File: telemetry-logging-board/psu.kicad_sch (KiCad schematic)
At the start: 23 parts, among them U10 TPS22919DCK, U16 TPS22919DCK, U17 TPS22919DCK, U18 AP61300Z6, U8 AP61300Z6

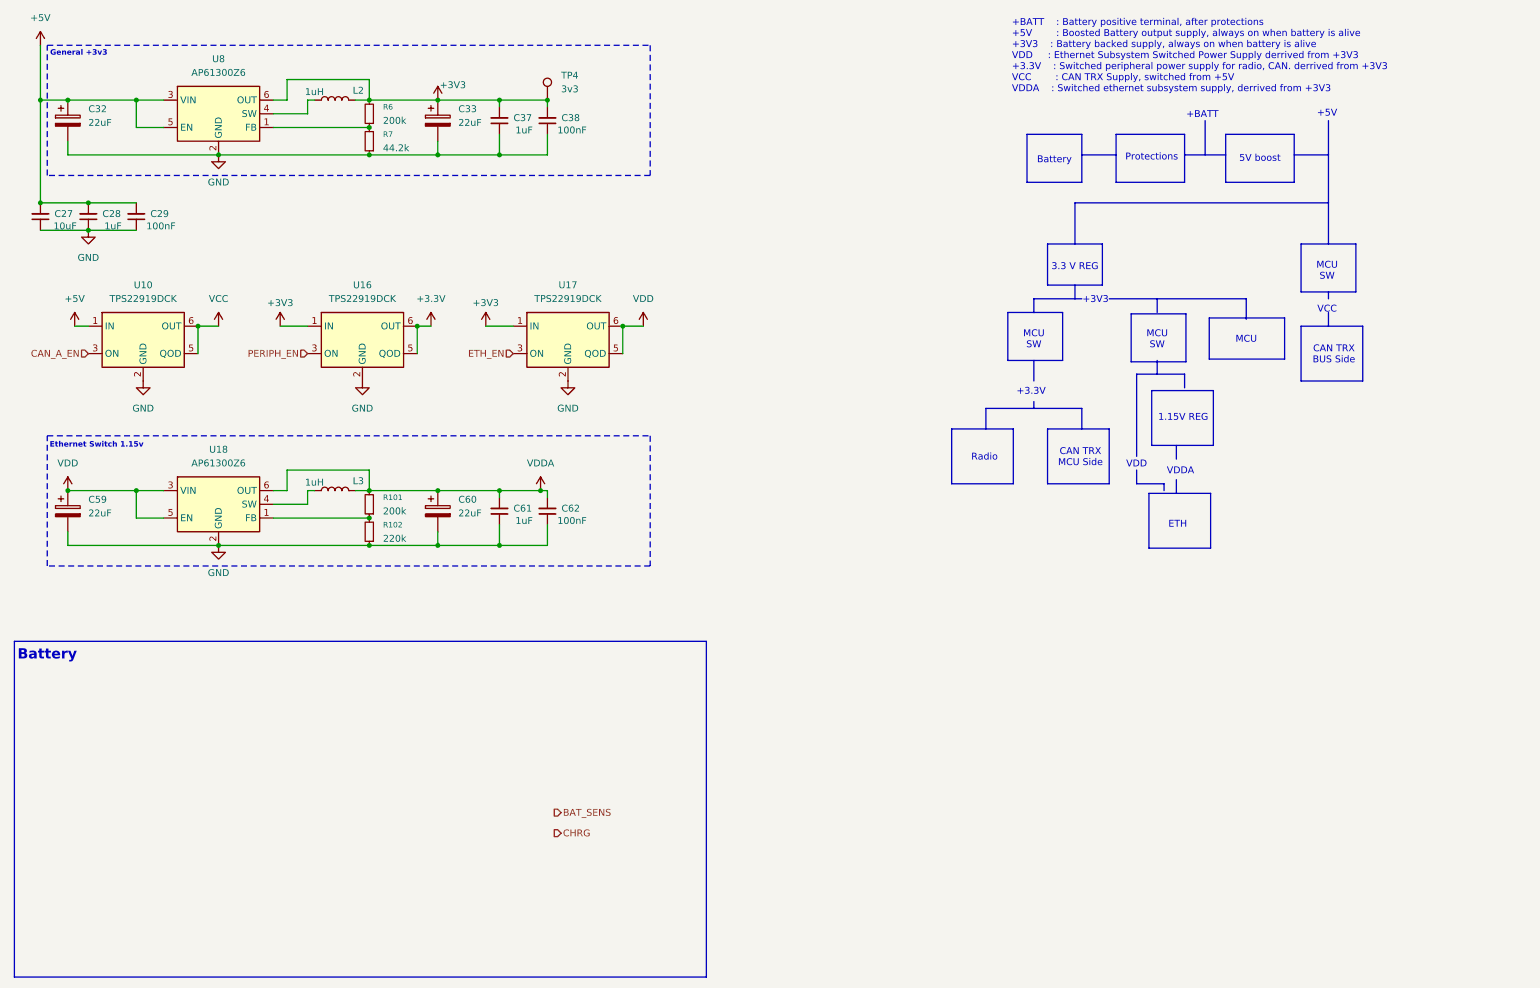
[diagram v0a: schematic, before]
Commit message: replace LR2021 with seeed wio LR2021, rework psu
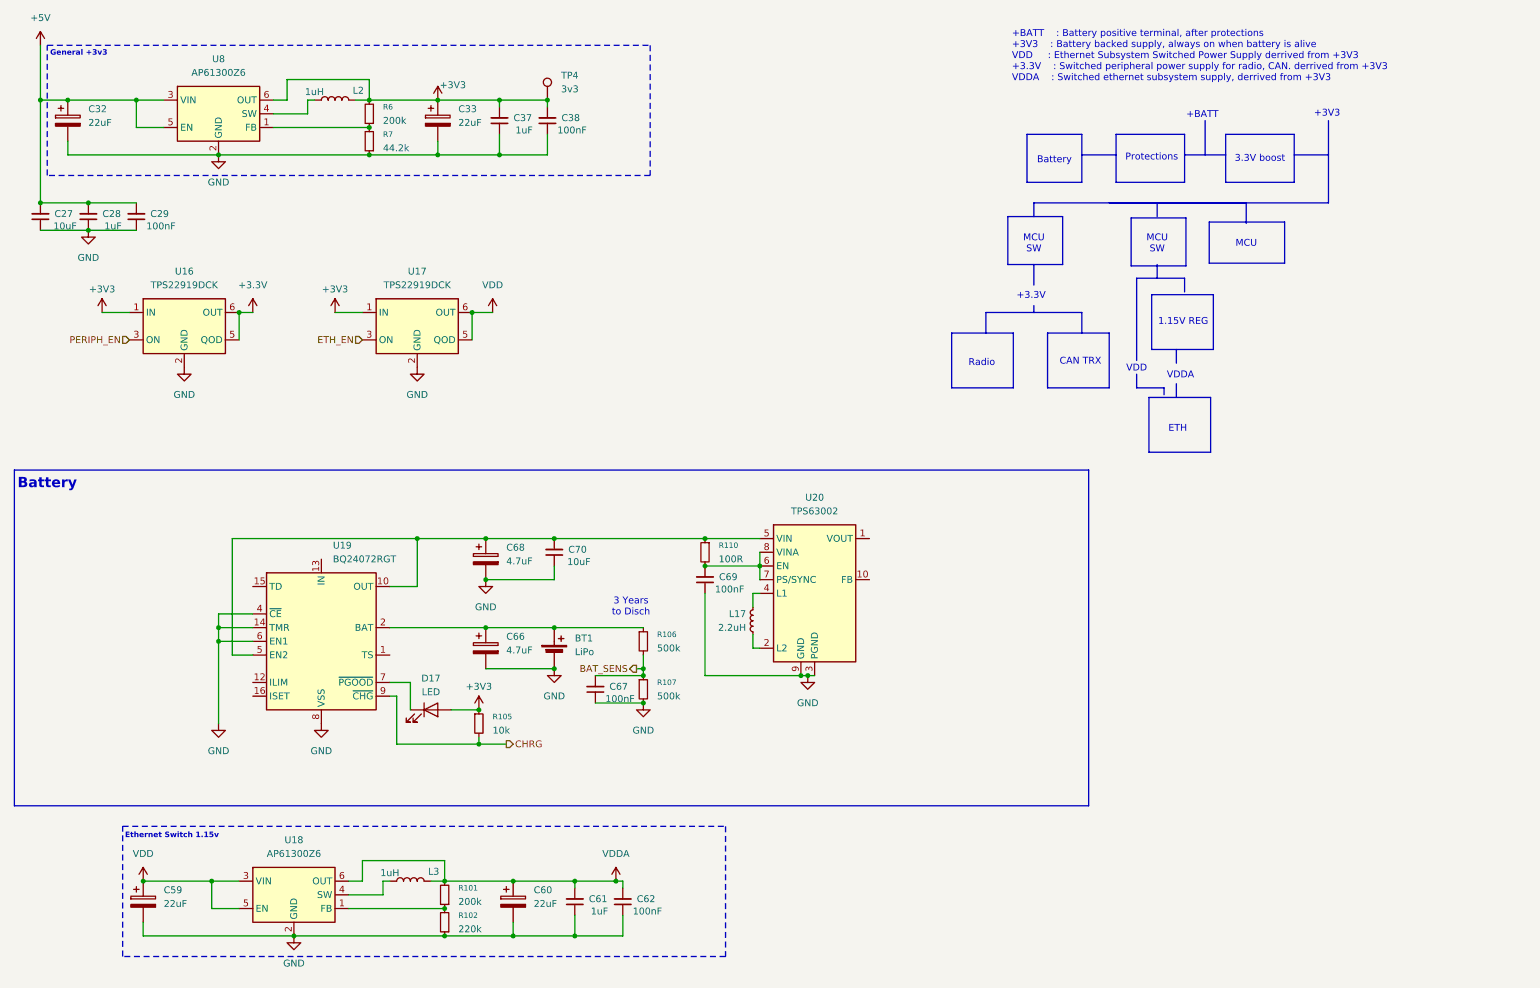
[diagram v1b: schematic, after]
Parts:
- removed U10: TPS22919DCK, Package_TO_SOT_SMD:SOT-363_SC-70-6, symbol Power_Management:TPS22919DCK
- added BT1: LiPo, symbol Device:Battery_Cell
- added C66, C68: 4.7uF, symbol Device:C_Polarized
- added C67, C69: 100nF, symbol Device:C_Small
- added C70: 10uF, symbol Device:C_Small
- added D17: LED, symbol Device:LED
- added L17: 2.2uH, symbol Device:L_Small
- added R105: 10k, symbol Device:R_Small
- added R106, R107: 500k, symbol Device:R_Small
- added R110: 100R, symbol Device:R_Small
- added U19: BQ24072RGT, Package_DFN_QFN:VQFN-16-1EP_3x3mm_P0.5mm_EP1.6x1.6mm, symbol Battery_Management:BQ24072RGT
- added U20: TPS63002, Package_SON:Texas_DRC0010J_ThermalVias, symbol Regulator_Switching:TPS63002
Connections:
- net +3V3: now also D17.2 (A), R105.1
- net BAT_SENS: now also C67.2, R106.2, R107.1
- net CHRG: now also R105.2, U19.9 (~{CHG})
- net GND: now also BT1.2 (-), C66.2, C67.1, C68.2, C69.1, C70.1, R107.2, U19.14 (TMR), U19.17 (VSS), U19.4 (~{CE}), U19.6 (EN1), U19.8 (VSS), U20.11 (PGND), U20.3 (PGND), U20.9 (GND)
- new net: C68.1, C70.2, R110.1, U19.10 (OUT), U19.11 (OUT), U19.5 (EN2), U20.5 (VIN)
- new net: C69.2, R110.2, U20.6 (EN), U20.7 (PS/SYNC), U20.8 (VINA)
- new net: L17.2, U20.2 (L2)
- new net: L17.1, U20.4 (L1)
- new net: BT1.1 (+), C66.1, R106.1, U19.2 (BAT), U19.3 (BAT)
- new net: D17.1 (K), U19.7 (~{PGOOD})
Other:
- note added: "+BATT : Battery positive terminal, after protections +3V3 : Battery backed supply, always on when battery is alive VDD : Ethernet Subsystem Switched Power Supply derrived from +3V3 +3.3V : Switched peripheral power supply for radio, CAN. derrived from +3V3 VDDA : Switched ethernet subsystem supply, derrived from +3V3"
- note added: "3 Years to Disch"
- note added: "3.3V boost"
- note added: "CAN TRX"
- note removed: "+5V"
- note removed: "+BATT : Battery positive terminal, after protections +5V : Boosted Battery output supply, always on when battery is alive +3V3 : Battery backed supply, always on when battery is alive VDD : Ethernet Subsystem Switched Power Supply derrived from +3V3 +3.3V : Switched peripheral power supply for radio, CAN. derrived from +3V3 VCC : CAN TRX Supply, switched from +5V VDDA : Switched ethernet subsyste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"
- note removed: "3.3 V REG"
- note removed: "5V boost"
- note removed: "CAN TRX BUS Side"
- note removed: "CAN TRX MCU Side"
- note removed: "VCC"
- moved on the sheet: C59, C60, C61, C62, L3, R101, R102, U16, U17, U18
